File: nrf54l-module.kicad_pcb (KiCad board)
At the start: 4 copper layers, 16 x 25 mm, 122 parts, among them SW1 TS24CA, U1 NRF54L15-QFAA-R, U2 XL-0201SURC, U3 TLV62569DBVR, U4 XL-0201SURC, U5 XL-0201SURC, X1 XL7EL89CKI-111YLC-32M

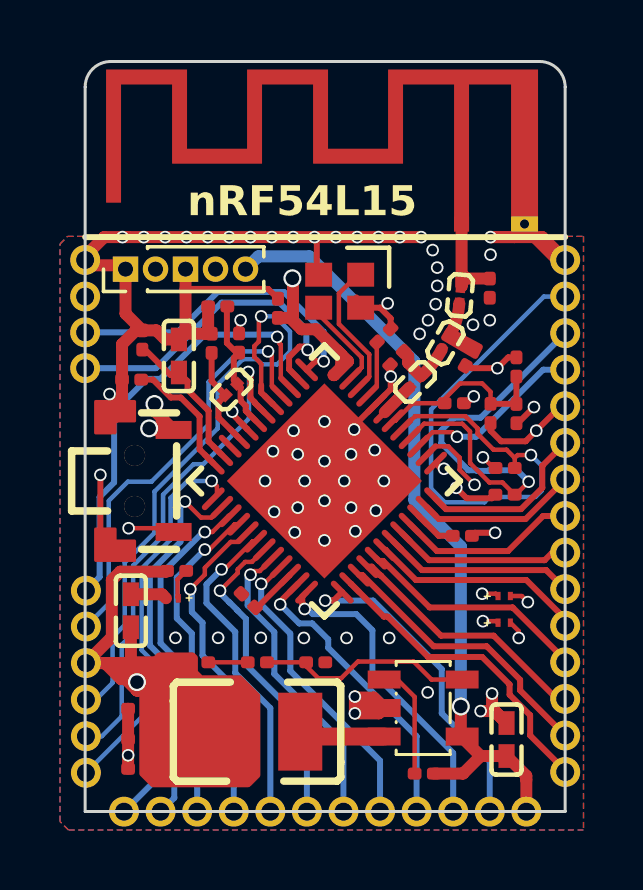
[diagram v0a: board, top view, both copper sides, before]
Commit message: chore: refactoring
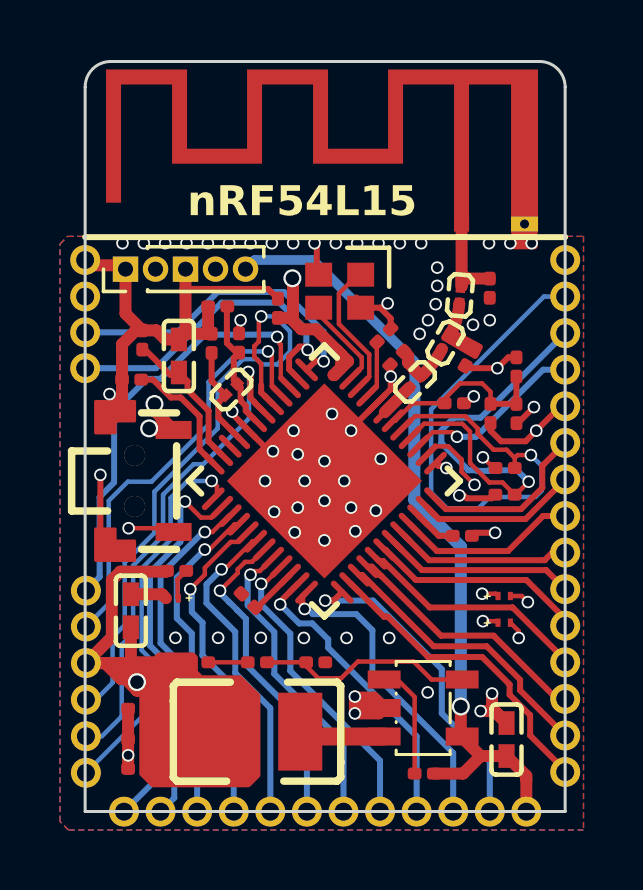
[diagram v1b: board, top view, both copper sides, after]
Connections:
- AE1 pad 2: (no net) -> GND
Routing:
- net GND: track 59.7 -> 45.9 mm, vias 67 -> 65
- net SWDIO: track 11.1 -> 12.1 mm
- net SWDCLK: track 17.7 -> 17.1 mm
